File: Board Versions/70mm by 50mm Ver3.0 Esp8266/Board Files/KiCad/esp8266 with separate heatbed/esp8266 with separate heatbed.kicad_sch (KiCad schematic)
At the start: 17 parts

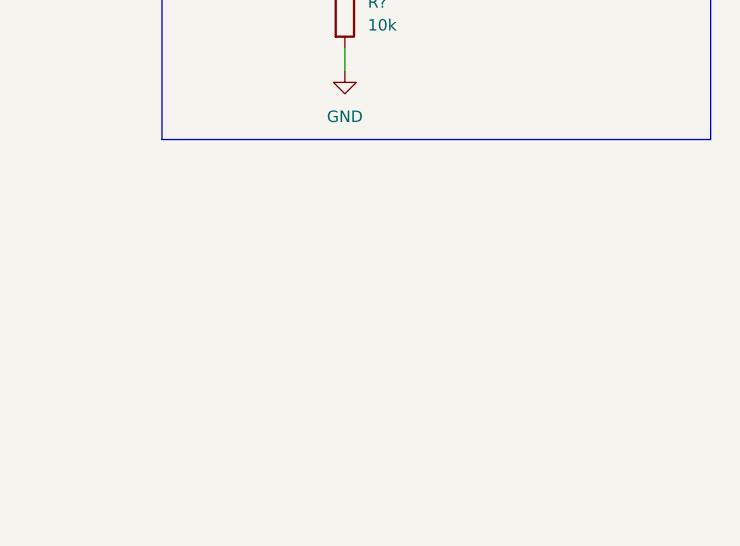
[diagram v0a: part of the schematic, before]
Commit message: Switches
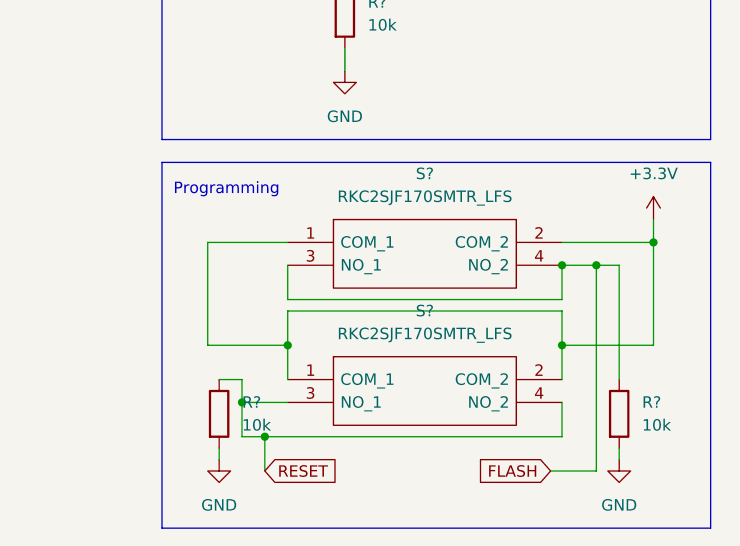
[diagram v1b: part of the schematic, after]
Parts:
- added R? (x2): 10k, symbol Device:R
- added S? (x2): RKC2SJF170SMTR_LFS, RKC2SJF170SMTRLFS, symbol library_loader:RKC2SJF170SMTR_LFS
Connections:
- net +3V3: now also S?.1 (COM_1), S?.1 (COM_1), S?.2 (COM_2), S?.2 (COM_2)
- net GND: now also R?.2, R?.2
- new net FLASH: R?.1, S?.3 (NO_1), S?.4 (NO_2)
- new net RESET: R?.1, S?.3 (NO_1), S?.4 (NO_2)
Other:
- note added: "Programming"
